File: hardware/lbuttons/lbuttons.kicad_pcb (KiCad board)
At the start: 2 copper layers, 107.7 x 55 mm, 7 parts, among them U1 SKRBAKE010, U2 SKRBAKE010, U3 SKRBAKE010, U4 SKRBAKE010, U5 SKRBAKE010

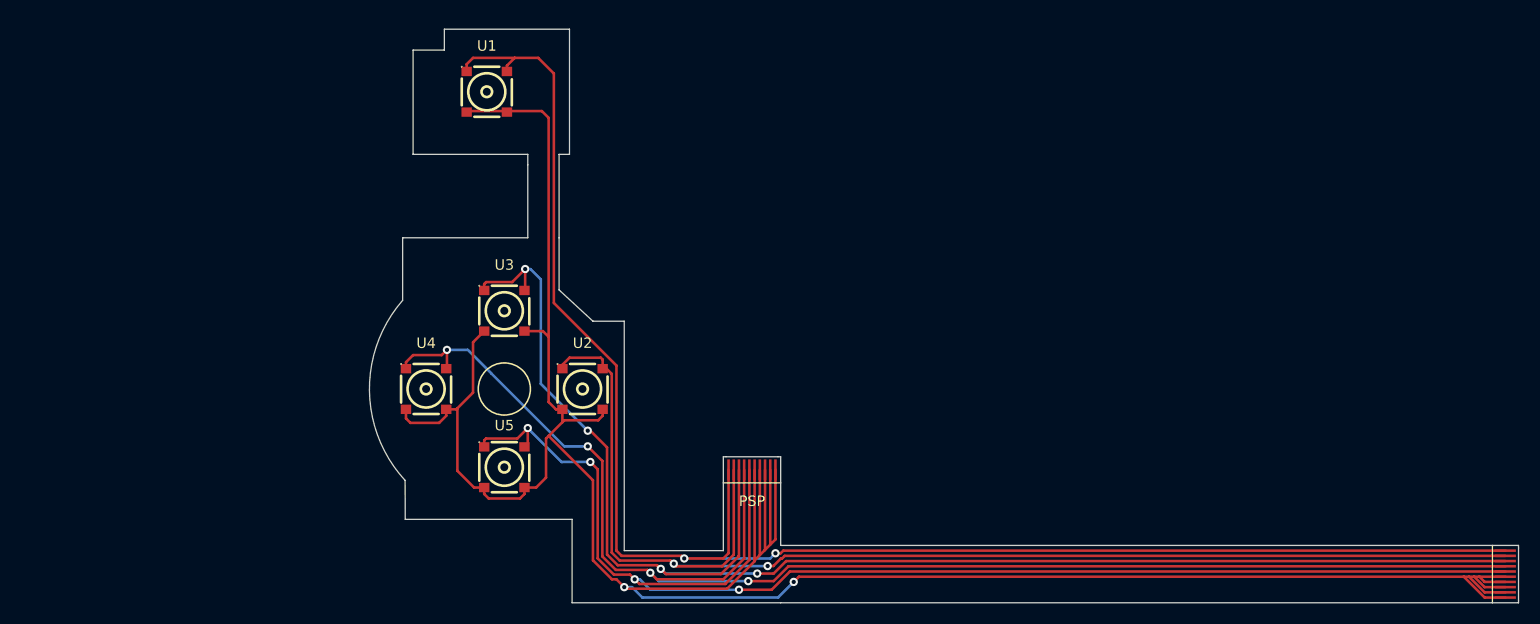
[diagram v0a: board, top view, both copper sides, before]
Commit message: Latest
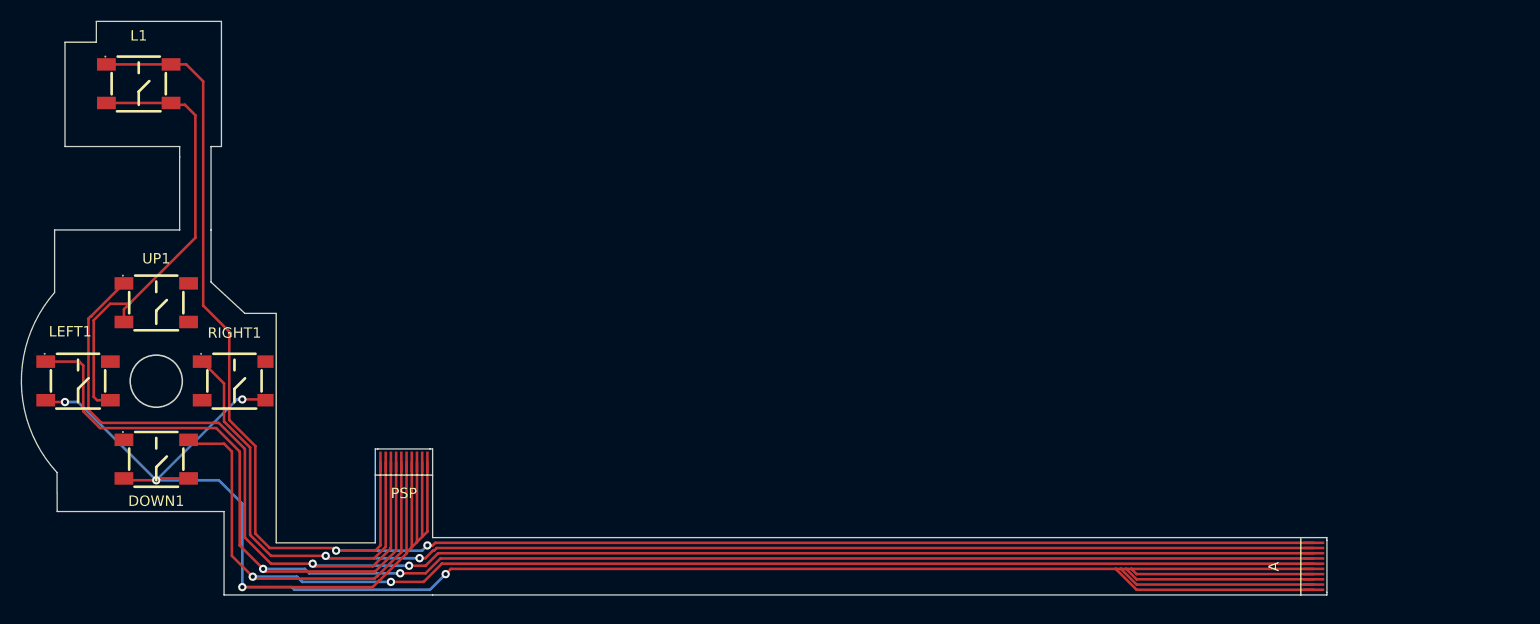
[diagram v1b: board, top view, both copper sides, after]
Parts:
- removed U1, U2, U3, U4, U5: SKRBAKE010, JLCPCB_footprint:KEY-SMD_4P-L4.0-W4.8-P3.90-LS4.8
- added DOWN1: K2-1187SQ-E4SW-06, JLCPCB_footprint:KEY-SMD_4P-L5.2-W5.2-P3.70-LS6.4, F.Cu at (91.1, 122.2)
- added L1: K2-1187SQ-E4SW-06, JLCPCB_footprint:KEY-SMD_4P-L5.2-W5.2-P3.70-LS6.4, F.Cu at (89.4, 86.2)
- added LEFT1: K2-1187SQ-E4SW-06, JLCPCB_footprint:KEY-SMD_4P-L5.2-W5.2-P3.70-LS6.4, F.Cu at (83.6, 114.8)
- added RIGHT1: K2-1187SQ-E4SW-06, JLCPCB_footprint:KEY-SMD_4P-L5.2-W5.2-P3.70-LS6.4, F.Cu at (98.6, 114.8)
- added UP1: K2-1187SQ-E4SW-06, JLCPCB_footprint:KEY-SMD_4P-L5.2-W5.2-P3.70-LS6.4, F.Cu at (91.1, 107.2)
- moved C3 33.4 mm to (115.1, 122.5)
- moved C4 18.4 mm to (202.1, 132.8)
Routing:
- net GND: track 257.8 -> 333.8 mm, vias 2 -> 5
- net /left: track 142.1 -> 160.6 mm, vias 4 -> 2
- net /up: track 142.4 -> 159.3 mm, vias 4 -> 2
- net /l1: track 158.1 -> 170.3 mm
- net /right: track 124.8 -> 136.3 mm
- net /down: track 134.5 -> 144.2 mm, vias 4 -> 2
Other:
- board size 107.7 x 55 mm -> 122.7 x 55 mm
- board text added: "A"
